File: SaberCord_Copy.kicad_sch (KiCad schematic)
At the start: 2 parts, among them J1 Conn_02x07_Counter_Clockwise, J3 USB_C_Receptacle

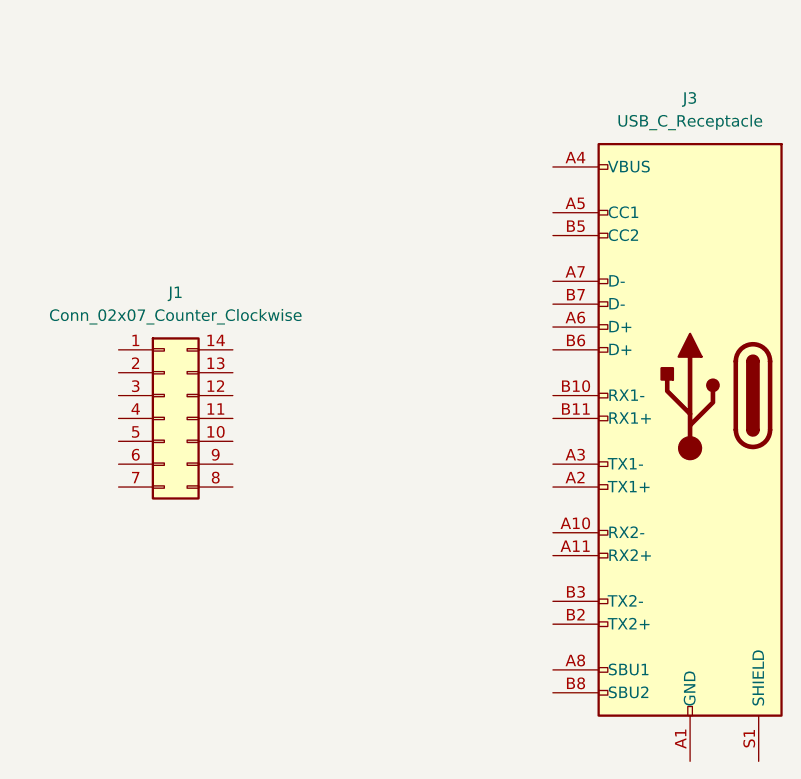
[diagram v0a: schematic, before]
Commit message: push before eod
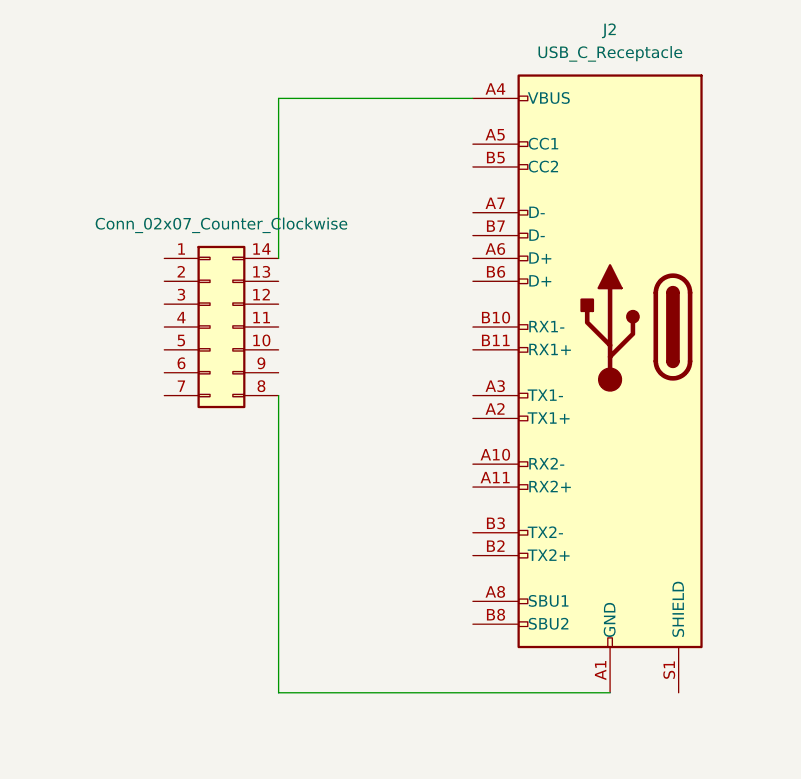
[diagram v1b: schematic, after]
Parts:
- removed J3: USB_C_Receptacle, Connector_USB:USB_C_Receptacle_Amphenol_12401610E4-2A_CircularHoles, symbol Connector:USB_C_Receptacle
- added J2: USB_C_Receptacle, Connector_USB:USB_C_Receptacle_Amphenol_12401548E4-2A_CircularHoles, symbol Connector:USB_C_Receptacle
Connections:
- net at J1.14 (Pin_14): now also J2.A4 (VBUS), J2.A9 (VBUS), J2.B4 (VBUS), J2.B9 (VBUS)
- net at J1.8 (Pin_8): now also J2.A1 (GND), J2.A12 (GND), J2.B1 (GND), J2.B12 (GND)
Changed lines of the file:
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@@
 (kicad_sch (version 20230121) (generator eeschema)
   (paper "A4")
-  (symbol (lib_id "Connector:USB_C_Receptacle") (at 207.01 85.09 0) (mirror y) (unit 1)
+  (wire (pts (xy 198.12 118.11) (xy 161.29 118.11))
+    (stroke (width 0) (type default))
+  )
+  (wire (pts (xy 161.29 52.07) (xy 161.29 69.85))
+    (stroke (width 0) (type default))
+  )
+  (wire (pts (xy 161.29 118.11) (xy 161.29 85.09))
+    (stroke (width 0) (type default))
+  )
+  (wire (pts (xy 182.88 52.07) (xy 161.29 52.07))
+    (stroke (width 0) (type default))
+  )
+  (symbol (lib_id "Connector:USB_C_Receptacle") (at 198.12 77.47 0) (mirror y) (unit 1)
     (in_bom yes) (on_board yes) (dnp no)
-    (property "Reference" "J3" (at 207.01 52.07 0)
+    (property "Reference" "J2" (at 198.12 44.45 0)
       (effects (font (size 1.27 1.27)))
     )
-    (property "Value" "USB_C_Receptacle" (at 207.01 54.61 0)
+    (property "Value" "USB_C_Receptacle" (at 198.12 46.99 0)
       (effects (font (size 1.27 1.27)))
     )
-    (property "Footprint" "Connector_USB:USB_C_Receptacle_Amphenol_12401610E4-2A_CircularHoles" (at 203.2 85.09 0)
+    (property "Footprint" "Connector_USB:USB_C_Receptacle_Amphenol_12401548E4-2A_CircularHoles" (at 194.31 77.47 0)
       (effects (font (size 1.27 1.27)) hide)
     )
-    (property "Datasheet" "https://www.usb.org/sites/default/files/documents/usb_type-c.zip" (at 203.2 85.09 0)
+    (property "Datasheet" "https://www.usb.org/sites/default/files/documents/usb_type-c.zip" (at 194.31 77.47 0)
       (effects (font (size 1.27 1.27)) hide)
     )
@@
       (project "SaberCord_Copy"
         (path "/be2c8e72-e310-467f-9e4e-b384214483bd"
-          (reference "J3") (unit 1)
+          (reference "J2") (unit 1)
         )
       )
     )
   )
-  (symbol (lib_id "Connector_Generic:Conn_02x07_Counter_Clockwise") (at 148.59 87.63 0) (unit 1)
+  (symbol (lib_id "Connector_Generic:Conn_02x07_Counter_Clockwise") (at 153.67 77.47 0) (unit 1)
     (in_bom yes) (on_board yes) (dnp no) (fields_autoplaced)
-    (property "Reference" "J1" (at 149.86 73.66 0)
+    (property "Reference" "J1" (at 154.94 63.5 0)
+      (effects (font (size 1.27 1.27)) hide)
+    )
+    (property "Value" "Conn_02x07_Counter_Clockwise" (at 154.94 66.04 0)
       (effects (font (size 1.27 1.27)))
     )
-    (property "Value" "Conn_02x07_Counter_Clockwise" (at 149.86 76.2 0)
-      (effects (font (size 1.27 1.27)))
-    )
-    (property "Footprint" "" (at 148.59 87.63 0)
+    (property "Footprint" "" (at 153.67 77.47 0)
       (effects (font (size 1.27 1.27)) hide)
     )
-    (property "Datasheet" "~" (at 148.59 87.63 0)
+    (property "Datasheet" "~" (at 153.67 77.47 0)
       (effects (font (size 1.27 1.27)) hide)
     )
